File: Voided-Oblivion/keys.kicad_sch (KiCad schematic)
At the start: 173 parts, among them U8 74AHCT125

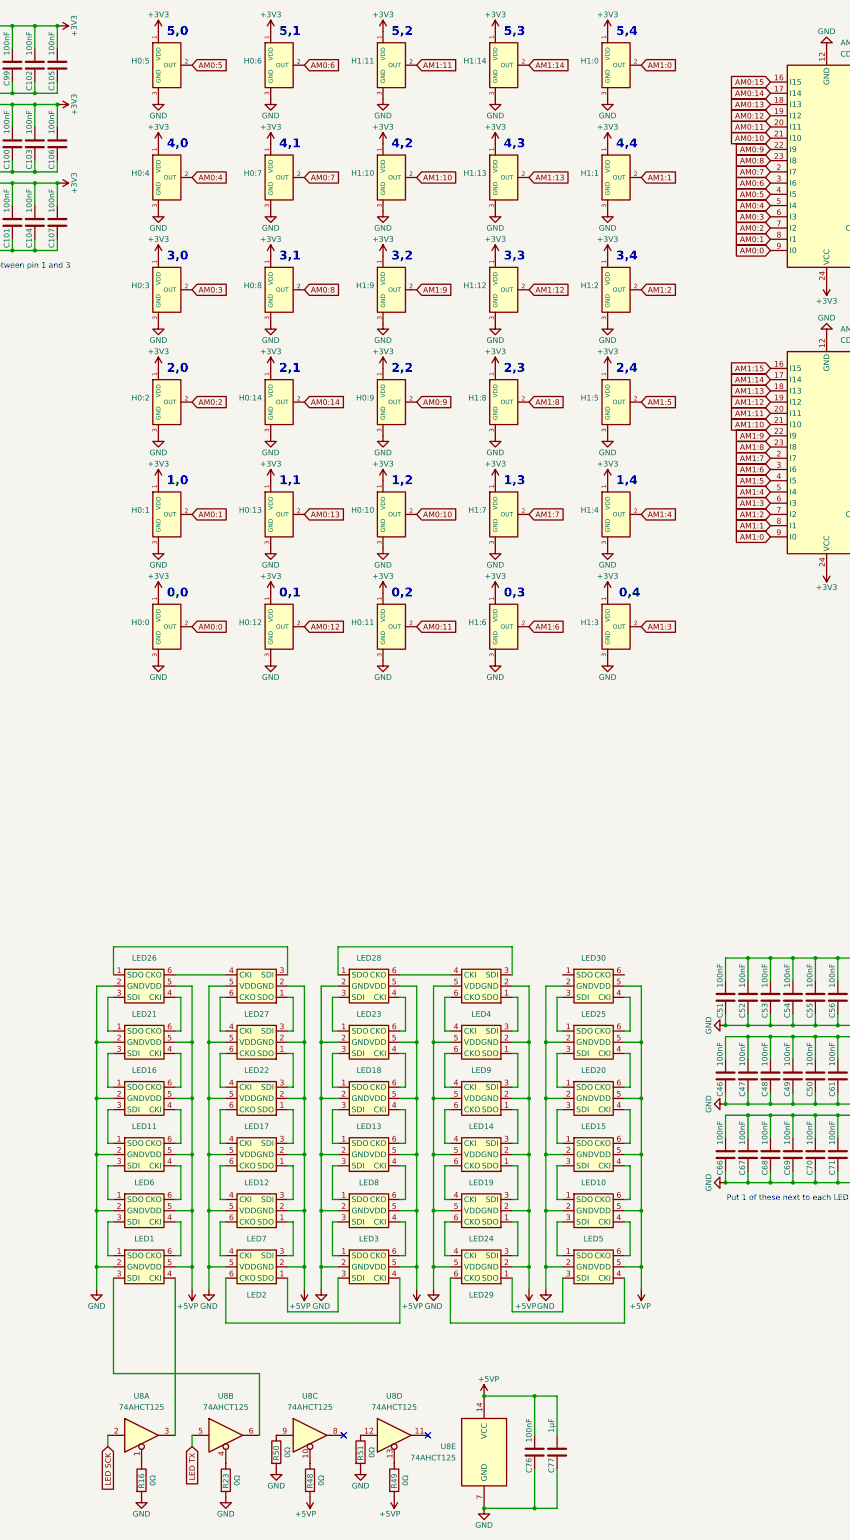
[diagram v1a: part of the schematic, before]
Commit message: update
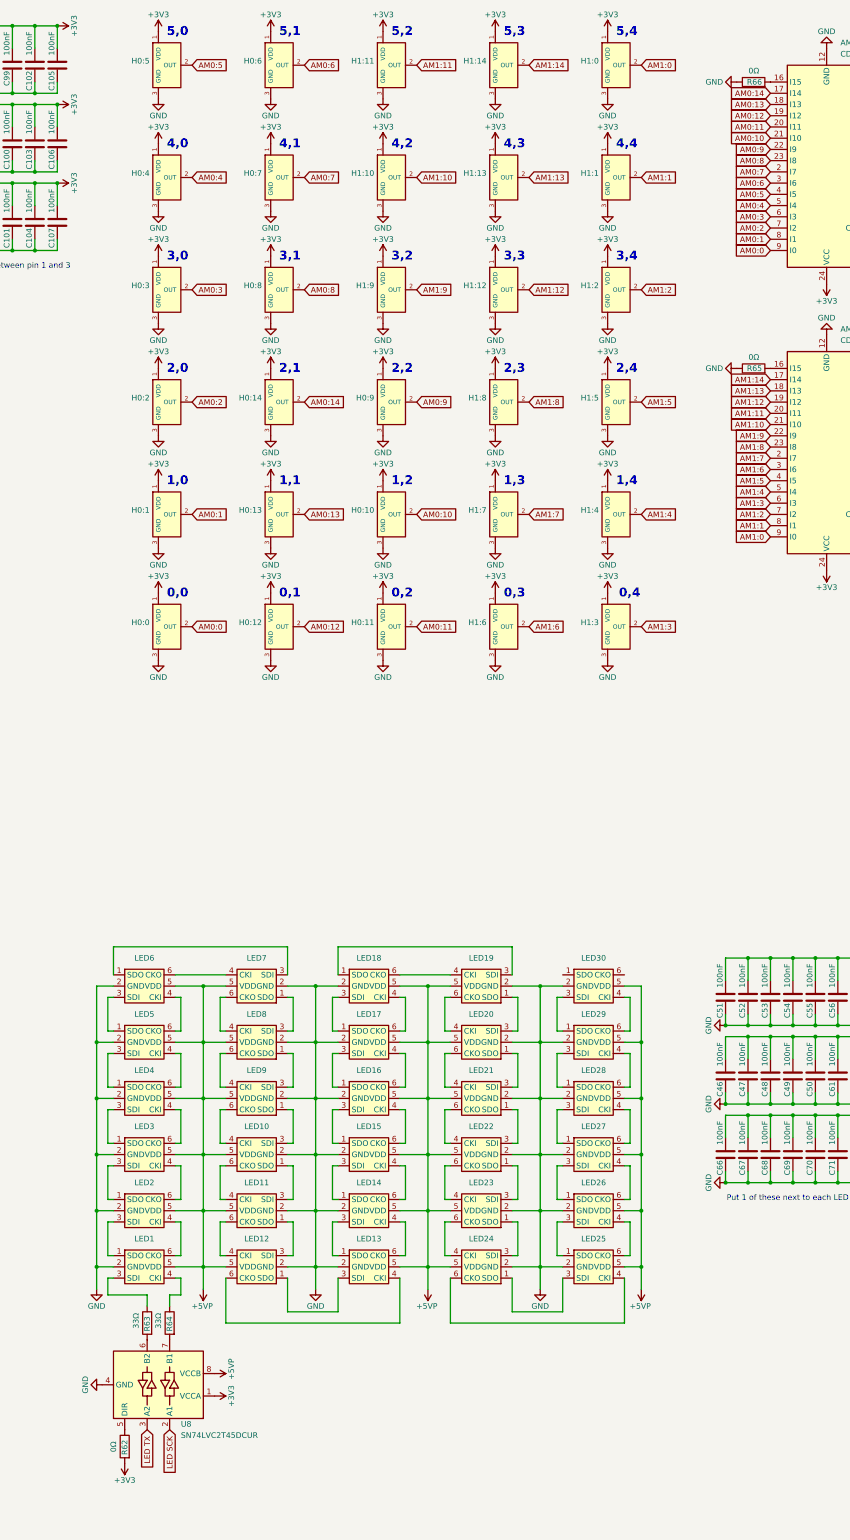
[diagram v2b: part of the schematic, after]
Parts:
- removed C76: 100nF, Capacitor_SMD:C_0402_1005Metric, symbol Device:C
- removed C77: 1µF, Capacitor_SMD:C_0402_1005Metric, symbol Device:C
- removed R16, R23, R48, R49, R50, R51: 0Ω, Resistor_SMD:R_0402_1005Metric, symbol Device:R
- removed U8: 74AHCT125, symbol 74xx:74AHCT125
- added R62, R65, R66: 0Ω, Resistor_SMD:R_0402_1005Metric, symbol Device:R
- added R63, R64: 33Ω, Resistor_SMD:R_0402_1005Metric, symbol Device:R
- added U8: SN74LVC2T45DCUR, Package_SO:VSSOP-8_2.3x2mm_P0.5mm, symbol Logic_LevelTranslator:SN74LVC2T45DCUR
- AM0, AM1: LCSC (none) -> C98457; MPN (none) -> CD74HC4067SM96; Manufacturer (none) -> Texas Instruments
- C100, C101, C102, C103, C104, C105, C106, C107, C108, C109, C46, C47, C48, C49, C50, C51, C52, C53, C54, C55, C56, C57, C58, C59, C60, C61, C62, C63, C64, C65, C66, C67, C68, C69, C70, C71, C72, C73, C74, C75, C78, C79, C80, C81, C82, C83, C84, C85, C86, C87, C88, C89, C90, C91, C92, C93, C94, C95, C96, C97, C98, C99: LCSC (none) -> C307331; MPN (none) -> CL05B104KB54PNC; Manufacturer (none) -> Samsung Electro-Mechanics
- H0:0, H0:1, H0:10, H0:11, H0:12, H0:13, H0:14, H0:2, H0:3, H0:4, H0:5, H0:6, H0:7, H0:8, H0:9, H1:0, H1:1, H1:10, H1:11, H1:12, H1:13, H1:14, H1:2, H1:3, H1:4, H1:5, H1:6, H1:7, H1:8, H1:9: LCSC (none) -> C266230; Manufacturer (none) -> GoChip Elec Tech (Shanghai)
- LED1, LED10, LED11, LED12, LED13, LED14, LED15, LED16, LED17, LED18, LED19, LED2, LED20, LED21, LED22, LED23, LED24, LED25, LED26, LED27, LED28, LED29, LED3, LED30, LED4, LED5, LED6, LED7, LED8, LED9: LCSC (none) -> C2909059; MPN (none) -> SK9822-EC20; Manufacturer (none) -> OPSCO Optoelectronics
- R52, R53, R54, R55, R56, R57, R58, R59, R60, R61: LCSC (none) -> C17168; MPN (none) -> 0402WGF0000TCE; Manufacturer (none) -> UNI-ROYAL
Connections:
- net +3V3: now also R62.2, U8.1 (VCCA)
- net +5VP: now also LED12.5 (VDD), LED14.5 (VDD), LED17.5 (VDD), LED19.5 (VDD), LED2.5 (VDD), LED22.5 (VDD), LED24.5 (VDD), LED27.5 (VDD), LED29.5 (VDD), LED4.5 (VDD), LED7.5 (VDD), LED9.5 (VDD), U8.8 (VCCB); no longer LED12.2 (GND), LED14.2 (GND), LED17.2 (GND), LED19.2 (GND), LED2.2 (GND), LED22.2 (GND), LED24.2 (GND), LED27.2 (GND), LED29.2 (GND), LED4.2 (GND), LED7.2 (GND), LED9.2 (GND)
- net GND: now also LED12.2 (GND), LED14.2 (GND), LED17.2 (GND), LED19.2 (GND), LED2.2 (GND), LED22.2 (GND), LED24.2 (GND), LED27.2 (GND), LED29.2 (GND), LED4.2 (GND), LED7.2 (GND), LED9.2 (GND), R65.1, R66.1, U8.4 (GND); no longer LED12.5 (VDD), LED14.5 (VDD), LED17.5 (VDD), LED19.5 (VDD), LED2.5 (VDD), LED22.5 (VDD), LED24.5 (VDD), LED27.5 (VDD), LED29.5 (VDD), LED4.5 (VDD), LED7.5 (VDD), LED9.5 (VDD)
- net LED SCK: now also U8.2 (A1)
- net LED TX: now also U8.3 (A2)
- net at LED8.1 (SDO): now also LED9.3 (SDI); no longer LED13.3 (SDI)
- net at LED8.3 (SDI): now also LED7.1 (SDO); no longer LED3.1 (SDO)
- net at LED8.4 (CKI): now also LED7.6 (CKO); no longer LED3.6 (CKO)
- net at LED8.6 (CKO): now also LED9.4 (CKI); no longer LED13.4 (CKI)
- net at LED13.1 (SDO): now also LED14.3 (SDI); no longer LED18.3 (SDI)
- net at LED13.6 (CKO): now also LED14.4 (CKI); no longer LED18.4 (CKI)
- net at LED14.1 (SDO): now also LED15.3 (SDI); no longer LED19.3 (SDI)
- net at LED9.1 (SDO): now also LED10.3 (SDI); no longer LED14.3 (SDI)
- net at LED9.6 (CKO): now also LED10.4 (CKI); no longer LED14.4 (CKI)
- net at LED14.6 (CKO): now also LED15.4 (CKI); no longer LED19.4 (CKI)
- net at LED30.3 (SDI): now also LED29.1 (SDO); no longer LED25.1 (SDO)
- net at LED30.4 (CKI): now also LED29.6 (CKO); no longer LED25.6 (CKO)
- net at LED12.1 (SDO): now also LED13.3 (SDI); no longer LED7.3 (SDI)
- net at LED12.3 (SDI): now also LED11.1 (SDO); no longer LED17.1 (SDO)
- net at LED12.4 (CKI): now also LED11.6 (CKO); no longer LED17.6 (CKO)
- net at LED12.6 (CKO): now also LED13.4 (CKI); no longer LED7.4 (CKI)
- net at LED2.3 (SDI): now also LED1.1 (SDO); no longer LED7.1 (SDO)
- net at LED2.4 (CKI): now also LED1.6 (CKO); no longer LED7.6 (CKO)
- net at LED21.1 (SDO): now also LED22.3 (SDI); no longer LED26.3 (SDI)
- net at LED21.3 (SDI): now also LED20.1 (SDO); no longer LED16.1 (SDO)
- net at LED21.4 (CKI): now also LED20.6 (CKO); no longer LED16.6 (CKO)
- net at LED21.6 (CKO): now also LED22.4 (CKI); no longer LED26.4 (CKI)
- net at LED28.1 (SDO): now also LED29.3 (SDI); no longer LED4.3 (SDI)
- net at LED28.3 (SDI): now also LED27.1 (SDO); no longer LED23.1 (SDO)
- net at LED28.4 (CKI): now also LED27.6 (CKO); no longer LED23.6 (CKO)
- net at LED28.6 (CKO): now also LED29.4 (CKI); no longer LED4.4 (CKI)
- net at LED19.1 (SDO): now also LED20.3 (SDI); no longer LED24.3 (SDI)
- net at LED19.6 (CKO): now also LED20.4 (CKI); no longer LED24.4 (CKI)
- net at LED5.1 (SDO): now also LED6.3 (SDI); no longer LED10.3 (SDI)
- net at LED5.3 (SDI): now also LED4.1 (SDO); no longer LED29.1 (SDO)
- net at LED5.4 (CKI): now also LED4.6 (CKO); no longer LED29.6 (CKO)
- net at LED5.6 (CKO): now also LED6.4 (CKI); no longer LED10.4 (CKI)
- net at LED16.3 (SDI): now also LED15.1 (SDO); no longer LED11.1 (SDO)
- net at LED11.3 (SDI): now also LED10.1 (SDO); no longer LED6.1 (SDO)
- net at LED11.4 (CKI): now also LED10.6 (CKO); no longer LED6.6 (CKO)
- net at LED16.4 (CKI): now also LED15.6 (CKO); no longer LED11.6 (CKO)
- net at LED1.3 (SDI): now also R63.1
- net at LED1.4 (CKI): now also R64.1
- net at LED25.3 (SDI): now also LED24.1 (SDO); no longer LED20.1 (SDO)
- net at LED25.4 (CKI): now also LED24.6 (CKO); no longer LED20.6 (CKO)
- net at LED17.3 (SDI): now also LED16.1 (SDO); no longer LED22.1 (SDO)
- net at LED17.4 (CKI): now also LED16.6 (CKO); no longer LED22.6 (CKO)
- net at LED18.1 (SDO): now also LED19.3 (SDI); no longer LED23.3 (SDI)
- net at LED18.6 (CKO): now also LED19.4 (CKI); no longer LED23.4 (CKI)
- net AM0:15: no longer names the net of AM0.16 (I15)
- net AM0:15: now also R66.2
- net AM1:15: no longer names the net of AM1.16 (I15)
- net AM1:15: now also R65.2
- new net: R63.2, U8.6 (B2)
- new net: R64.2, U8.7 (B1)
- new net: LED6.1 (SDO), LED7.3 (SDI)
- new net: LED6.6 (CKO), LED7.4 (CKI)
- new net: LED25.1 (SDO), LED26.3 (SDI)
- new net: LED25.6 (CKO), LED26.4 (CKI)
- new net: LED23.1 (SDO), LED24.3 (SDI)
- new net: LED23.6 (CKO), LED24.4 (CKI)
- new net: LED22.1 (SDO), LED23.3 (SDI)
- new net: LED22.6 (CKO), LED23.4 (CKI)
- new net: LED3.1 (SDO), LED4.3 (SDI)
- new net: LED3.6 (CKO), LED4.4 (CKI)
- new net: R62.1, U8.5 (DIR)
- new net: LED17.1 (SDO), LED18.3 (SDI)
- new net: LED17.6 (CKO), LED18.4 (CKI)
- no-connect marks 2 -> 0
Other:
- moved on the sheet: LED10, LED11, LED12, LED13, LED14, LED15, LED16, LED17, LED18, LED19, LED2, LED20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

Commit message: i think the schematic is acctualy done this time, (besides little tiny things)
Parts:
- AM0, AM1: LCSC C98457 -> (none); MPN CD74HC4067SM96 -> (none); Manufacturer Texas Instruments -> (none)
- C100, C101, C102, C103, C104, C105, C106, C107, C108, C109, C46, C47, C48, C49, C50, C51, C52, C53, C54, C55, C56, C57, C58, C59, C60, C61, C62, C63, C64, C65, C66, C67, C68, C69, C70, C71, C72, C73, C74, C75, C78, C79, C80, C81, C82, C83, C84, C85, C86, C87, C88, C89, C90, C91, C92, C93, C94, C95, C96, C97, C98, C99: LCSC C307331 -> (none); MPN CL05B104KB54PNC -> (none); Manufacturer Samsung Electro-Mechanics -> (none)
- H0:0, H0:1, H0:10, H0:11, H0:12, H0:13, H0:14, H0:2, H0:3, H0:4, H0:5, H0:6, H0:7, H0:8, H0:9, H1:0, H1:1, H1:10, H1:11, H1:12, H1:13, H1:14, H1:2, H1:3, H1:4, H1:5, H1:6, H1:7, H1:8, H1:9: LCSC C266230 -> (none); Manufacturer GoChip Elec Tech (Shanghai) -> (none)
- LED1, LED10, LED11, LED12, LED13, LED14, LED15, LED16, LED17, LED18, LED19, LED2, LED20, LED21, LED22, LED23, LED24, LED25, LED26, LED27, LED28, LED29, LED3, LED30, LED4, LED5, LED6, LED7, LED8, LED9: LCSC C2909059 -> (none); MPN SK9822-EC20 -> (none); Manufacturer OPSCO Optoelectronics -> (none)
- R52, R53, R54, R55, R56, R57, R58, R59, R60, R61, R62, R65, R66: LCSC C17168 -> (none); MPN 0402WGF0000TCE -> (none); Manufacturer UNI-ROYAL -> (none)
- R63, R64: LCSC C138002 -> (none); MPN RC0402FR-0733RL -> (none); Manufacturer Yageo -> (none)
- U8: LCSC C15741 -> (none); MPN SN74LVC2T45DCUR -> (none); Manufacturer Texas Instruments -> (none)
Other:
- note added: "Alignment Footprints"
- note added: "Analog Mux"
- note added: "Hall Effect Sensors"
- note added: "RGB LEDs"
- moved on the sheet: C100, C101, C102, C103, C104, C105, C106, C107, C46, C47, C48, C49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

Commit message: drc rules and stuff
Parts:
- AM0, AM1: LCSC (none) -> C98457; MPN (none) -> CD74HC4067SM96; Manufacturer (none) -> Texas Instruments
- C100, C101, C102, C103, C104, C105, C106, C107, C108, C109, C46, C47, C48, C49, C50, C51, C52, C53, C54, C55, C56, C57, C58, C59, C60, C61, C62, C63, C64, C65, C66, C67, C68, C69, C70, C71, C72, C73, C74, C75, C78, C79, C80, C81, C82, C83, C84, C85, C86, C87, C88, C89, C90, C91, C92, C93, C94, C95, C96, C97, C98, C99: LCSC (none) -> C307331; MPN (none) -> CL05B104KB54PNC; Manufacturer (none) -> Samsung Electro-Mechanics
- H0:0, H0:1, H0:10, H0:11, H0:12, H0:13, H0:14, H0:2, H0:3, H0:4, H0:5, H0:6, H0:7, H0:8, H0:9, H1:0, H1:1, H1:10, H1:11, H1:12, H1:13, H1:14, H1:2, H1:3, H1:4, H1:5, H1:6, H1:7, H1:8, H1:9: LCSC (none) -> C266230; LCSC Part C266230 -> (none); Manufacturer (none) -> GoChip Elec Tech (Shanghai)
- LED1, LED10, LED11, LED12, LED13, LED14, LED15, LED16, LED17, LED18, LED19, LED2, LED20, LED21, LED22, LED23, LED24, LED25, LED26, LED27, LED28, LED29, LED3, LED30, LED4, LED5, LED6, LED7, LED8, LED9: LCSC (none) -> C2909059; MPN (none) -> SK9822-EC20; Manufacturer (none) -> OPSCO Optoelectronics
- R52, R53, R54, R55, R56, R57, R58, R59, R60, R61, R62, R65, R66: LCSC (none) -> C17168; MPN (none) -> 0402WGF0000TCE; Manufacturer (none) -> UNI-ROYAL(Uniroyal Elec)
- R63, R64: LCSC (none) -> C138002; MPN (none) -> RC0402FR-0733RL; Manufacturer (none) -> YAGEO
- U8: LCSC (none) -> C15741; MPN (none) -> SN74LVC2T45DCUR; Manufacturer (none) -> Texas Instruments

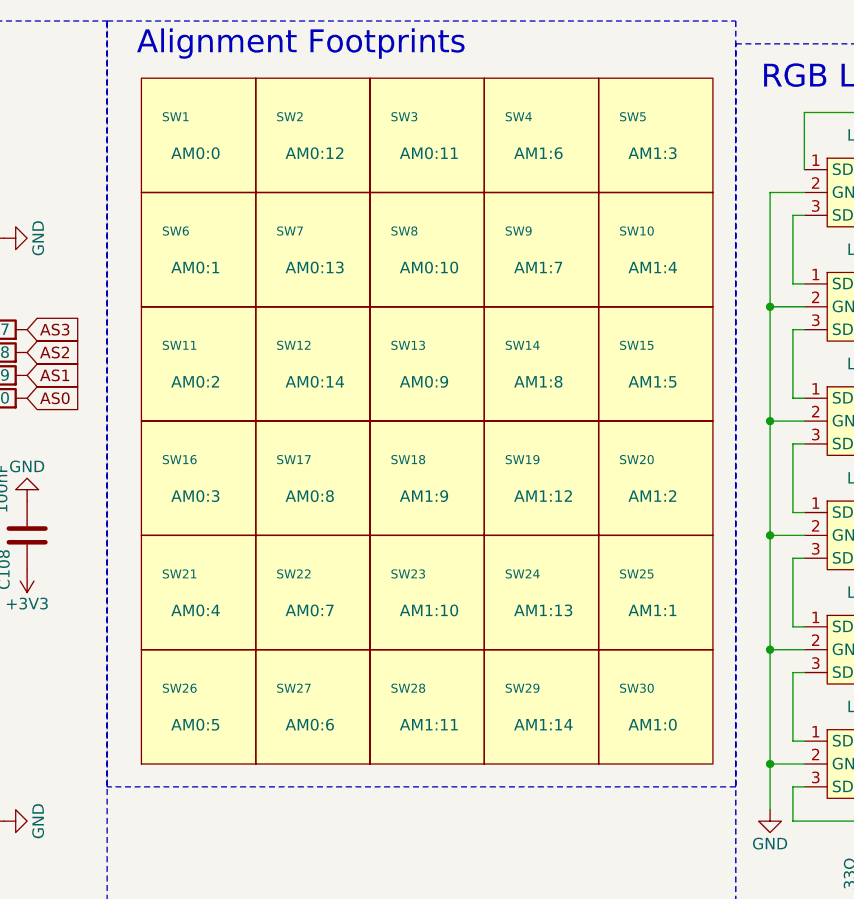
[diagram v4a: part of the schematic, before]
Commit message: blaaa why does placeing and routing things take so looonnggggggggg >:c
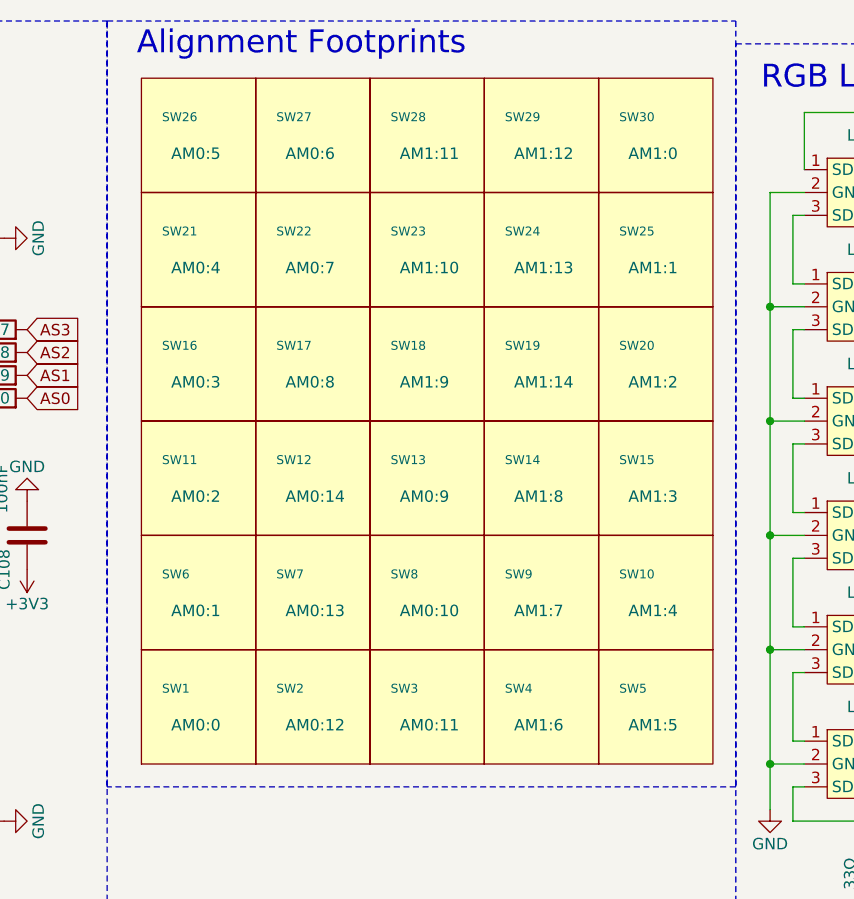
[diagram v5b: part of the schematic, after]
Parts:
- renumbered AM1:14 to AM1:12, AM1:12 to AM1:14, AM1:5 to AM1:3, AM1:3 to AM1:5
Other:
- moved on the sheet: AM0:0, AM0:1, AM0:10, AM0:11, AM0:12, AM0:13, AM0:14, AM0:2, AM0:3, AM0:4, AM0:5, AM0:6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
